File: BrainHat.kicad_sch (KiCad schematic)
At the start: 47 parts, among them J1 Power, J2 Output, J3 Electrodes, J4 Status, U1 AD8232, U2 ADS1115IDGS, U3 TS5A3159ADBVR, U4 SN74LV1T34DBV, U5 SN74LV1T34DBV

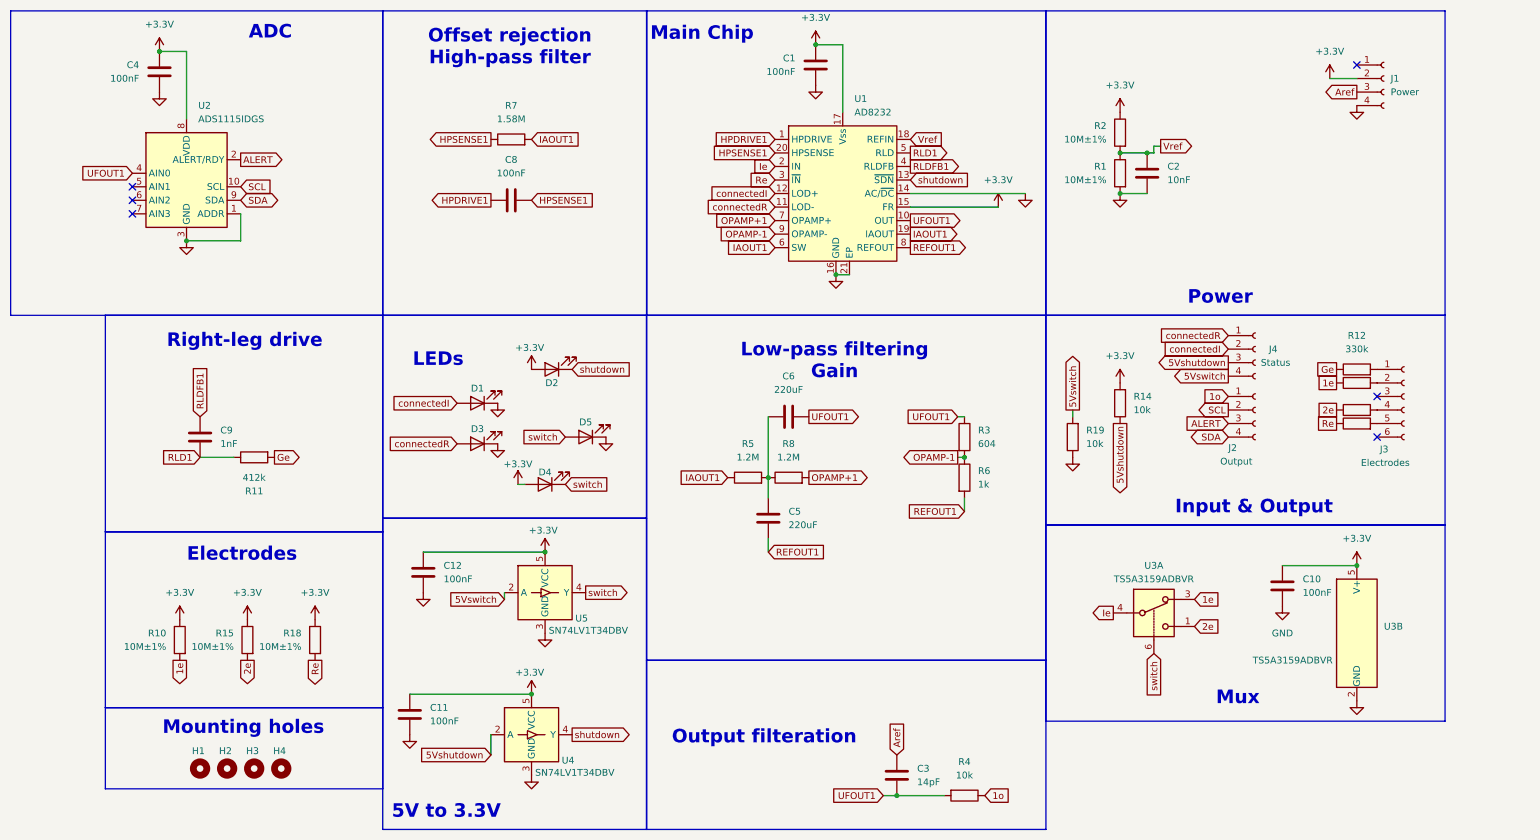
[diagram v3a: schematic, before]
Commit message: Redid PCB again
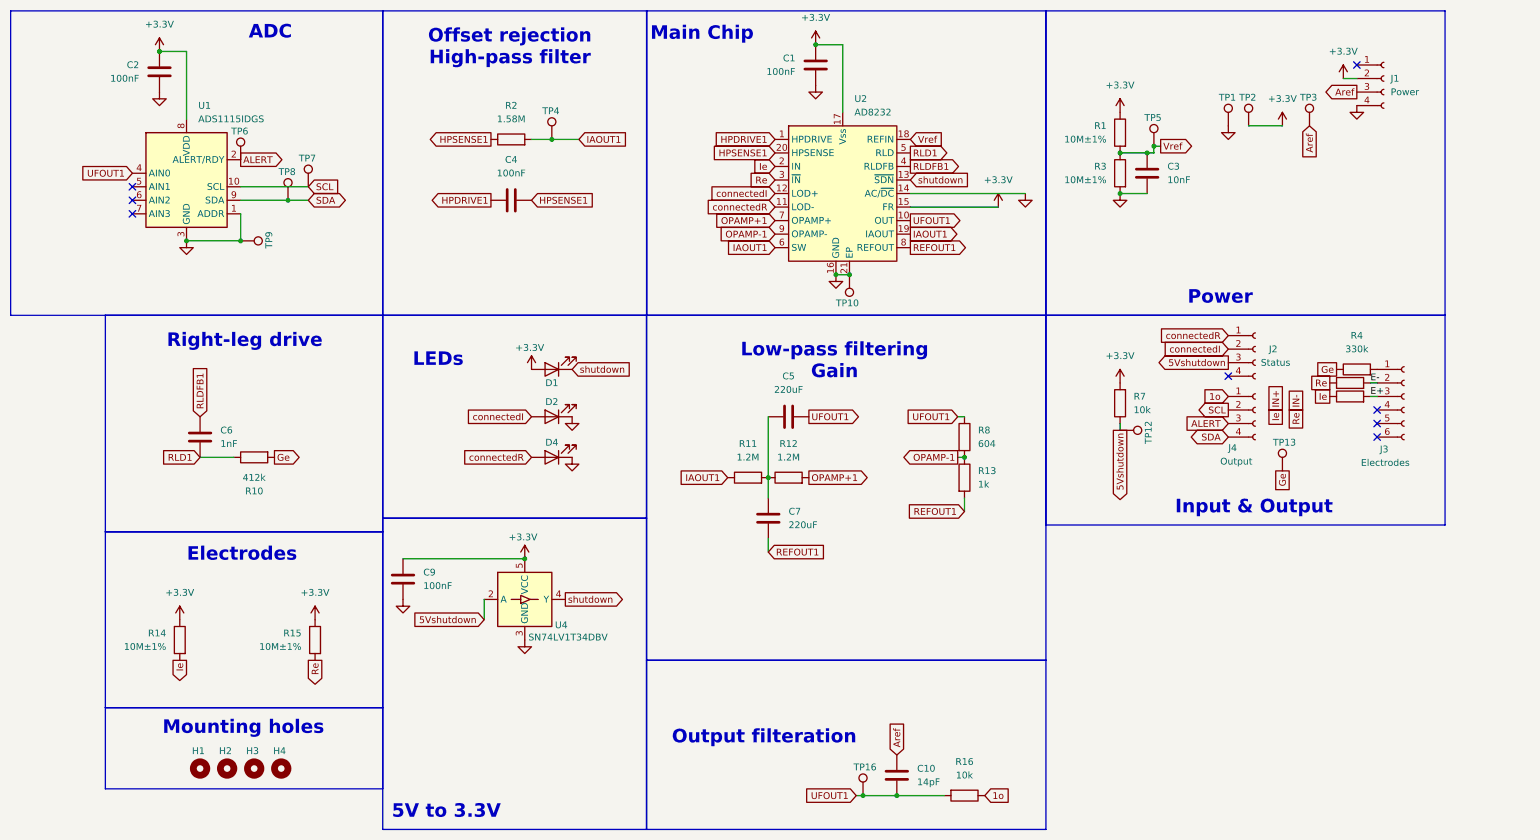
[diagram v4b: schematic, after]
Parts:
- removed C10, C12: 100nF, Capacitor_SMD:C_1210_3225Metric, symbol Device:C
- removed D4, D5: XL-1608UGC-04, LED_SMD:LED_0603_1608Metric, symbol Device:LED
- removed R13, R16, R17: 330k, Resistor_SMD:R_0402_1005Metric, symbol Device:R
- removed R18, R2: 10M±1%, Resistor_THT:R_Axial_DIN0309_L9.0mm_D3.2mm_P15.24mm_Horizontal, symbol Device:R
- removed R19: 10k, Resistor_SMD:R_1206_3216Metric, symbol Device:R
- removed U3: TS5A3159ADBVR, Package_TO_SOT_SMD:SOT-23-6, symbol Analog_Switch:TS5A3159ADBVR
- removed U5: SN74LV1T34DBV, Package_TO_SOT_SMD:SOT-23-5, symbol Logic_LevelTranslator:SN74LV1T34DBV
- added R3: 10M±1%, Resistor_SMD:R_0402_1005Metric, symbol Device:R
- added R5, R6: 330k, Resistor_SMD:R_0402_1005Metric, symbol Device:R
- added TP1, TP10, TP12, TP13, TP16, TP2, TP3, TP4, TP5, TP6, TP7, TP8, TP9: TestPoint, TestPoint:TestPoint_Pad_D1.5mm, symbol Connector:TestPoint
- C3: renamed from C2; footprint Capacitor_THT:C_Disc_D12.0mm_W4.4mm_P7.75mm -> Capacitor_SMD:C_0805_2012Metric; LCSC Part # C2896242 -> C569765
- C4: renamed from C8; footprint Capacitor_SMD:C_1210_3225Metric -> Capacitor_THT:C_Disc_D7.5mm_W5.0mm_P5.00mm; LCSC Part # C569766 -> C7502406
- R1, R15: footprint Resistor_THT:R_Axial_DIN0309_L9.0mm_D3.2mm_P15.24mm_Horizontal -> Resistor_SMD:R_0402_1005Metric; LCSC Part # C2979775 -> C2933065
- R10: renamed from R11; footprint Resistor_SMD:R_2010_5025Metric -> Resistor_SMD:R_0402_1005Metric; LCSC Part # C421836 -> C5126037
- R14: renamed from R10; footprint Resistor_THT:R_Axial_DIN0309_L9.0mm_D3.2mm_P15.24mm_Horizontal -> Resistor_SMD:R_0402_1005Metric; LCSC Part # C2979775 -> C2933065
- renumbered C3 to C10, C4 to C2, C6 to C5, C9 to C6, C5 to C7, C11 to C9, D2 to D1, D1 to D2, D3 to D4, J4 to J2, J2 to J4, R5 to R11, R8 to R12, R6 to R13, R4 to R16, R7 to R2, R12 to R4, R14 to R7, R3 to R8, U2 to U1, U1 to U2
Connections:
- net Ie is gone; now on net IN+: U2.2 (IN)
- net Re is gone; now on net IN-: U2.3 (~{IN})
- net +3.3V: now also R1.1, TP2.1
- net 5Vshutdown: now also TP12.1
- net ALERT: now also TP6.1
- net Aref: now also TP3.1
- net GND: now also R3.2, TP1.1, TP10.1, TP9.1; no longer R1.2
- net Ge: now also TP13.1
- net IAOUT1: now also TP4.1
- net SCL: now also TP7.1
- net SDA: now also TP8.1
- net UFOUT1: now also TP16.1
- net Vref: now also R1.2, R3.1, TP5.1; no longer R1.1
- net E-: now reaches J3.2 (Pin_2)
- net E-: now also R5.2
- net E+: now reaches J3.3 (Pin_3)
- net E+: now also R6.2
- net 1e renamed IN+
- net IN+: now also R6.1
- net 2e renamed IN-
- net IN-: now also R5.1
- net 5Vswitch: no longer names the net of J2.4 (Pin_4)
- no-connect marks 6 -> 8
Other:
- note removed: "Mux"
- moved on the sheet: C9, D2, D4, U4
